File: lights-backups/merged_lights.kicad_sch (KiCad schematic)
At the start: 45 parts, among them J1 AVR-ISP-6, J2 Conn_01x02, J3 Conn_01x02, J4 Conn_01x02, J5 Conn_01x02, J6 Conn_01x02, Q1 AO3400A, Q2 IRLML2803, Q3 IRLML2803, Q4 IRLML2803, Q5 IRLML2803, Q6 AO3400A, Q7 AO3400A, Q8 AO3400A, SW1 SW_Push, U1 ATmega328P-A, U2 ADXL345

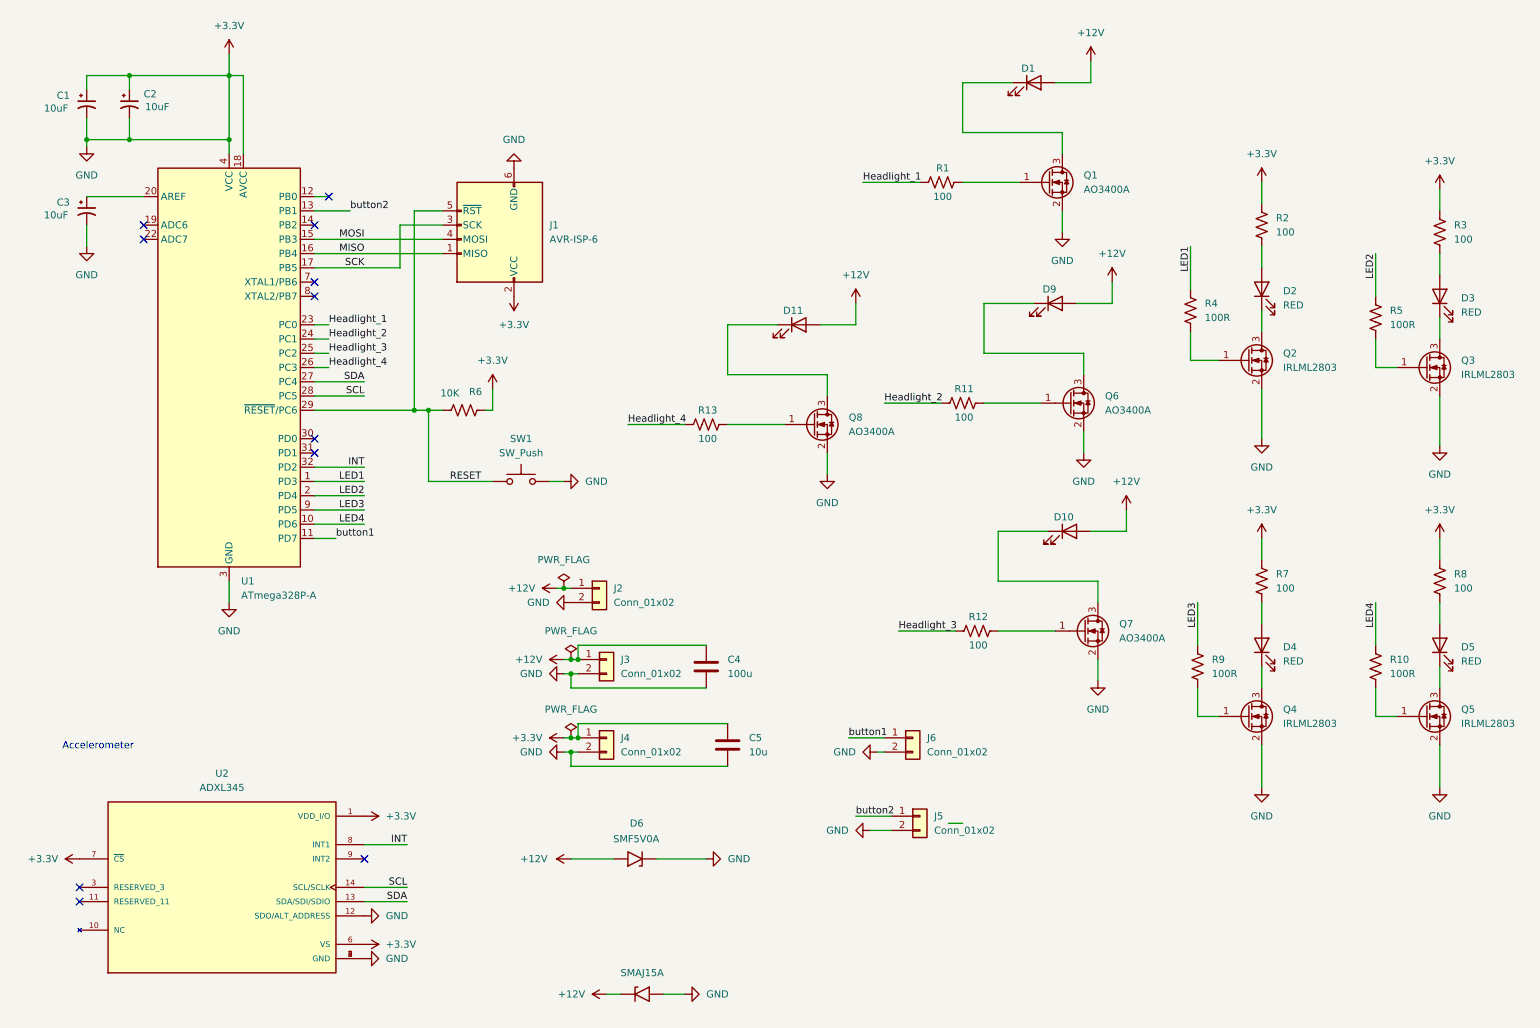
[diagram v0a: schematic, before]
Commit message: made updates with footprints and structure of schematic
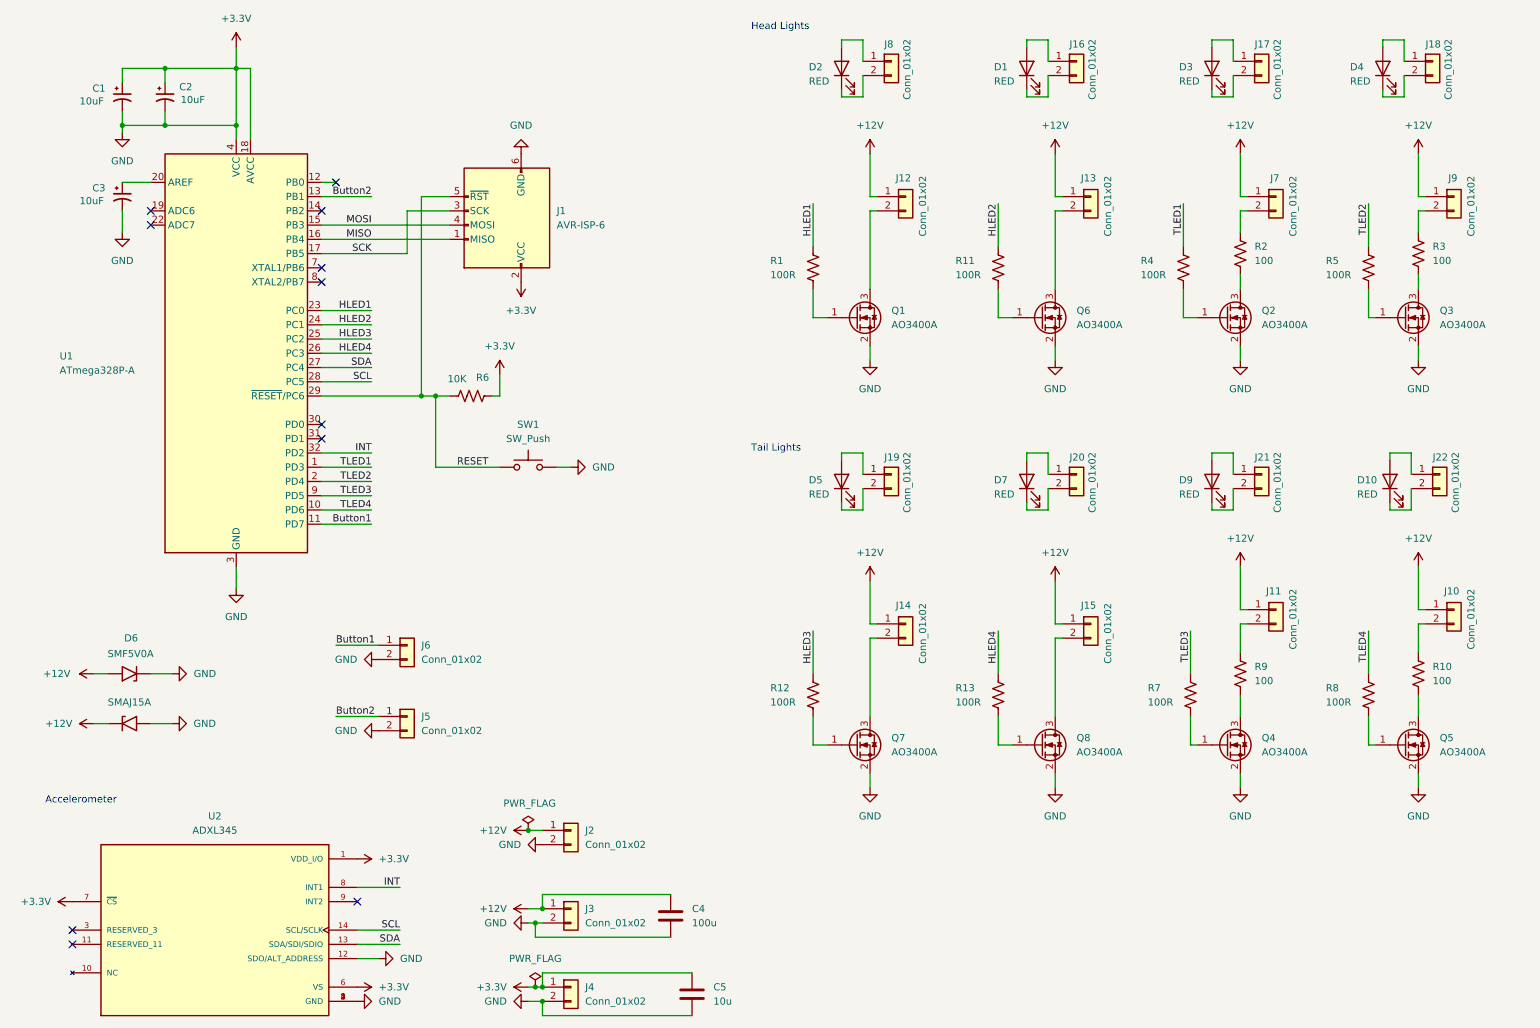
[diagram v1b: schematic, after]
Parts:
- removed D11: ~, symbol Device:LED
- removed Q2, Q3, Q4, Q5: IRLML2803, Package_TO_SOT_SMD:SOT-23, symbol Transistor_FET:IRLML2060
- added D7: RED, AB-EZD03-RA3:ABEZD03RA3, symbol Device:LED
- added J10, J11, J12, J13, J14, J15, J16, J17, J18, J19, J20, J21, J22, J7, J8, J9: Conn_01x02, Connector_JST:JST_PH_B2B-PH-K_1x02_P2.00mm_Vertical, symbol Connector_Generic:Conn_01x02
- added Q2, Q3, Q4, Q5: AO3400A, Package_TO_SOT_SMD:SOT-23, symbol Transistor_FET:AO3400A
- D1: value ~ -> RED; footprint (none) -> AB-EZD10C-A3-K65:ABEZD10CA3K65
- D10, D9: value ~ -> RED; footprint (none) -> AB-EZD03-RA3:ABEZD03RA3
- D2, D3, D4: footprint (none) -> AB-EZD10C-A3-K65:ABEZD10CA3K65
- D5: footprint (none) -> AB-EZD03-RA3:ABEZD03RA3
- J5, J6: footprint (none) -> Connector_JST:JST_PH_B2B-PH-K_1x02_P2.00mm_Vertical
- R1, R12, R7, R8: value 100 -> 100R
- R10, R9: value 100R -> 100
- R11, R13: value 100 -> 100R; footprint Resistor_SMD:R_0805_2012Metric_Pad1.20x1.40mm_HandSolder -> (none)
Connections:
- net +12V: now also J10.1 (Pin_1), J11.1 (Pin_1), J12.1 (Pin_1), J13.1 (Pin_1), J14.1 (Pin_1), J15.1 (Pin_1), J7.1 (Pin_1), J9.1 (Pin_1); no longer D1.2 (A), D10.2 (A), D9.2 (A)
- net +3.3V: now also Q2.2 (S), Q3.2 (S), Q4.2 (S), Q5.2 (S); no longer R2.1, R3.1, R7.1, R8.1
- net at D10.1 (K): now also J22.2 (Pin_2); no longer Q7.3 (D)
- net at Q6.3 (D): now also J13.2 (Pin_2); no longer D9.1 (K)
- net at R9.2: now also Q4.3 (D)
- net at R10.2: now also Q5.3 (D)
- net at D5.1 (K): now also J19.2 (Pin_2)
- net at R5.2: now also Q3.1 (G)
- net at D2.1 (K): now also J8.2 (Pin_2)
- net at D2.2 (A): now also J8.1 (Pin_1); no longer R2.2
- net at R8.2: now also Q5.1 (G); no longer D5.2 (A)
- net at R7.2: now also Q4.1 (G); no longer D4.2 (A)
- net at Q8.3 (D): now also J15.2 (Pin_2)
- net at D3.1 (K): now also J17.2 (Pin_2)
- net at R3.2: now also Q3.3 (D); no longer D3.2 (A)
- net at D4.1 (K): now also J18.2 (Pin_2)
- net at R4.2: now also Q2.1 (G)
- net at D1.1 (K): now also J16.2 (Pin_2); no longer Q1.3 (D)
- net Headlight_1 renamed HLED1
- net Headlight_2 renamed HLED2
- net Headlight_3 renamed HLED3
- net Headlight_4 renamed HLED4
- net LED1 renamed TLED1
- net LED2 renamed TLED2
- net LED3: no longer names the net of R9.1
- net LED3: now also J11.2 (Pin_2); no longer U1.9 (PD5)
- net LED4: no longer names the net of R10.1
- net LED4: now also J10.2 (Pin_2); no longer U1.10 (PD6)
- net button1 renamed Button1
- net button2 renamed Button2
- new net: D10.2 (A), J22.1 (Pin_1)
- new net: D5.2 (A), J19.1 (Pin_1)
- new net: D4.2 (A), J18.1 (Pin_1)
- new net: J14.2 (Pin_2), Q7.3 (D)
- new net: J7.2 (Pin_2), R2.1
- new net: Q2.3 (D), R2.2
- new net: D1.2 (A), J16.1 (Pin_1)
- new net: D9.1 (K), J21.2 (Pin_2)
- new net: D9.2 (A), J21.1 (Pin_1)
- new net: D7.2 (A), J20.1 (Pin_1)
- new net: D7.1 (K), J20.2 (Pin_2)
- new net: J9.2 (Pin_2), R3.1
- new net: J12.2 (Pin_2), Q1.3 (D)
- new net: D3.2 (A), J17.1 (Pin_1)
- new net TLED3: R7.1, U1.9 (PD5)
- new net TLED4: R8.1, U1.10 (PD6)
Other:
- note added: "Head Lights"
- note added: "Tail Lights"
- moved on the sheet: C1, C2, C3, C4, C5, D2, D6, J1, J2, J3, J4, J5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
